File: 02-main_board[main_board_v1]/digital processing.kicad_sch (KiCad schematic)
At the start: 19 parts, among them U5 PT61018PEL, U6 RCLAMP3354S_TCT, U7 ATA6561-GAQW-N, U8 74LVC4245APW_118

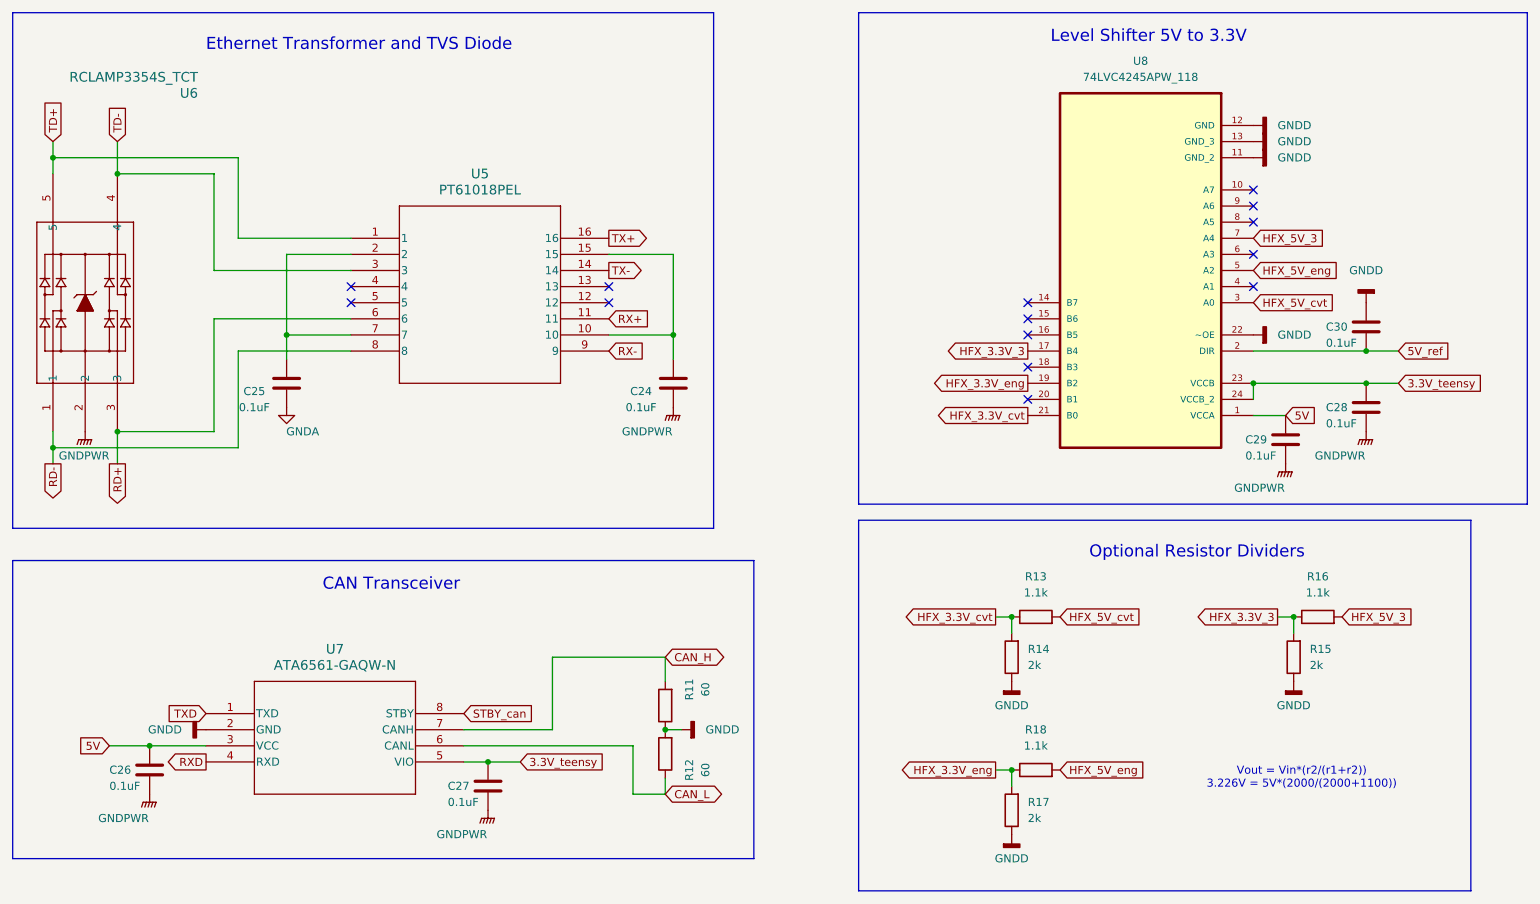
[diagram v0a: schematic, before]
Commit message: Updated with changes from PDR
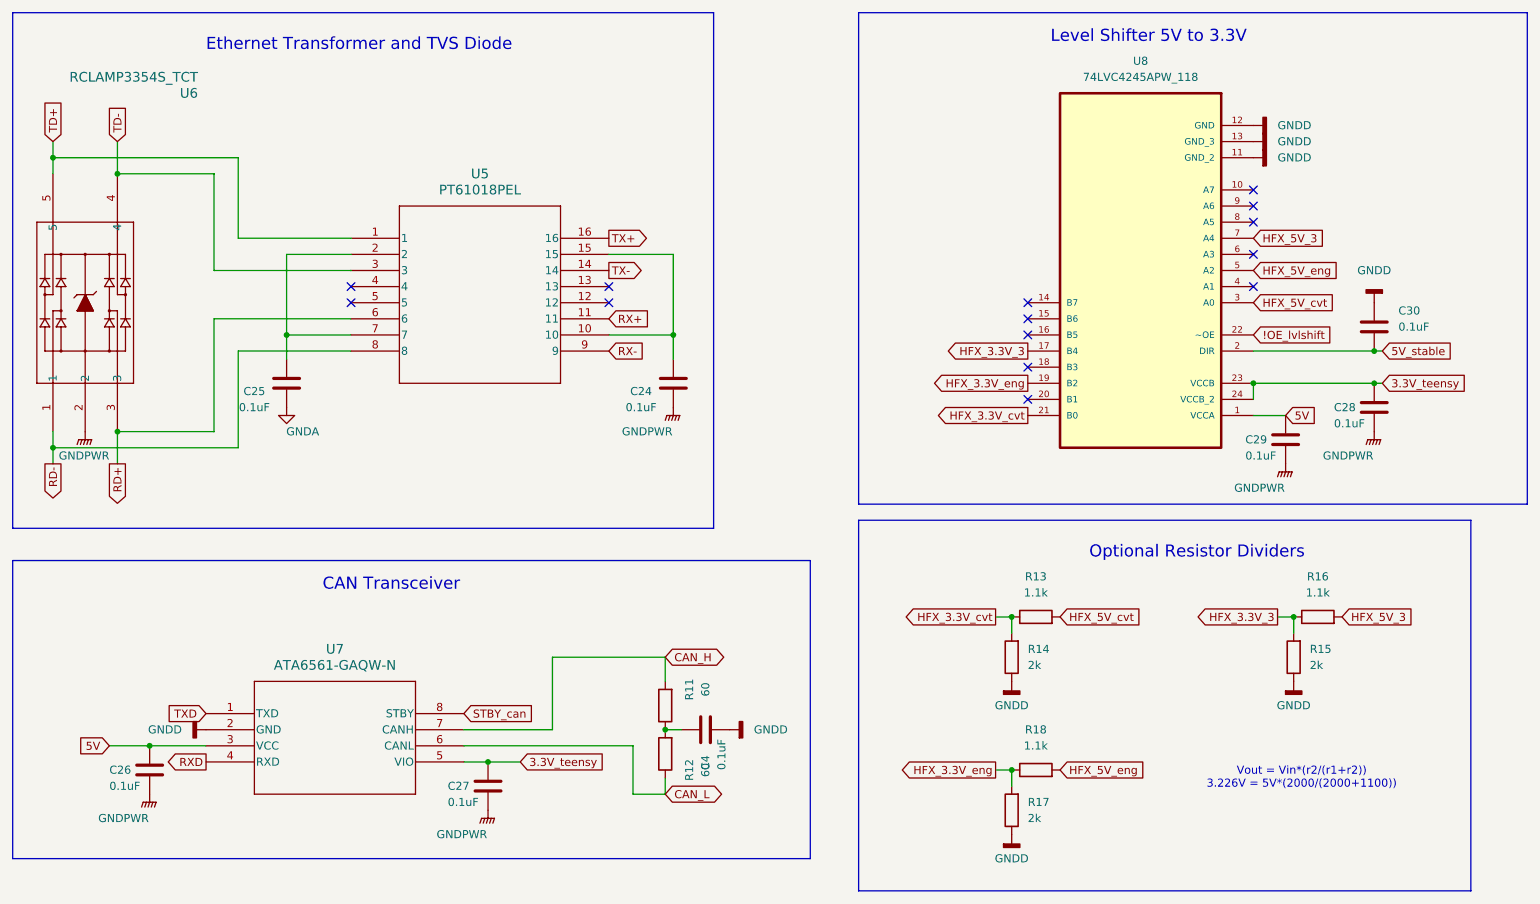
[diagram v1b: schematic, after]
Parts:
- added C4: 0.1uF, symbol Device:C
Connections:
- net GNDD: now also C4.1; no longer R11.1, R12.2, U8.22 (~OE)
- net 5V_ref renamed 5V_stable
- new net: C4.2, R11.1, R12.2
- new net !OE_lvlshift: U8.22 (~OE)
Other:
- moved on the sheet: C28, C30
